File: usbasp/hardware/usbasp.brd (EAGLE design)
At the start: 34.9 x 16.5 mm, 25 parts, among them IC1 ATMEGA8-16A, Q2 12Mhz, X1 USB-A-H

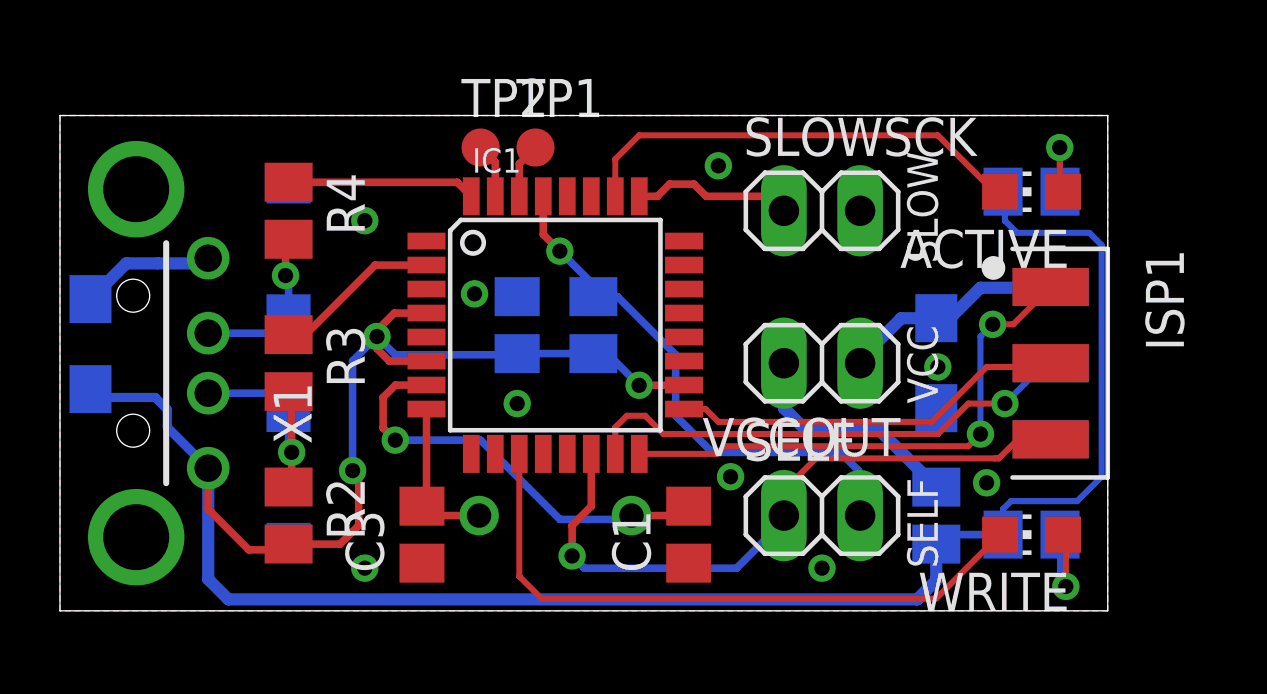
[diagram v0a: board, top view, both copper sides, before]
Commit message: many updates
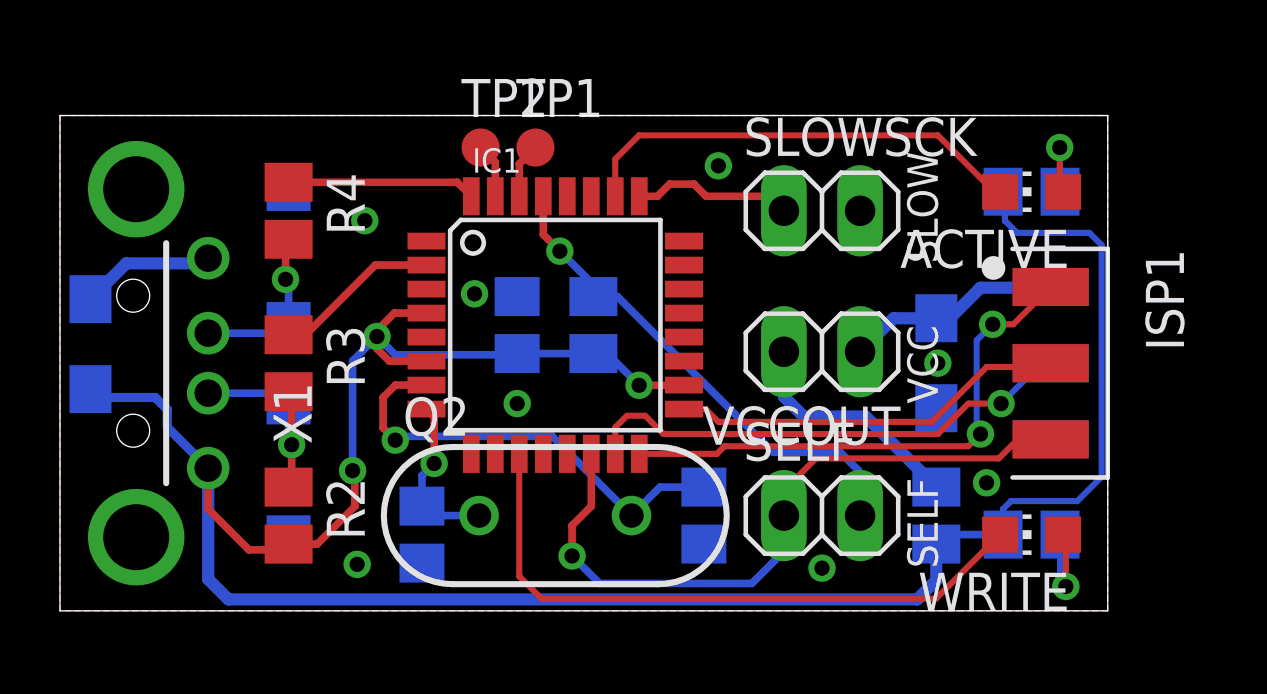
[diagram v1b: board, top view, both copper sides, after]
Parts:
- moved C1 0.81 mm to (21.5, 3.17), flipped to the bottom
- moved VCCOUT 0.38 mm to (25.4, 8.64)
- moved D1 0.25 mm to (7.62, 11.8)
- moved D2 0.25 mm to (7.62, 4.70)
- flipped C3 to the bottom
- flipped Q2 to the top, turned to 0 degrees
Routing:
- net SELFPROG: track 18.0 -> 16.8 mm
- net RESET: track 22.2 -> 23.2 mm
- net XTAL1: track 14.3 -> 15.0 mm
- net VCC: track 83.6 -> 83.0 mm
- net XTAL2: track 5.33 -> 5.54 mm, vias 0 -> 1
- net GND: vias 9 -> 8
